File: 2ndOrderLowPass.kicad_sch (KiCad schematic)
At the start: 14 parts, among them U2 LM2904DR, U3 LM2904DR

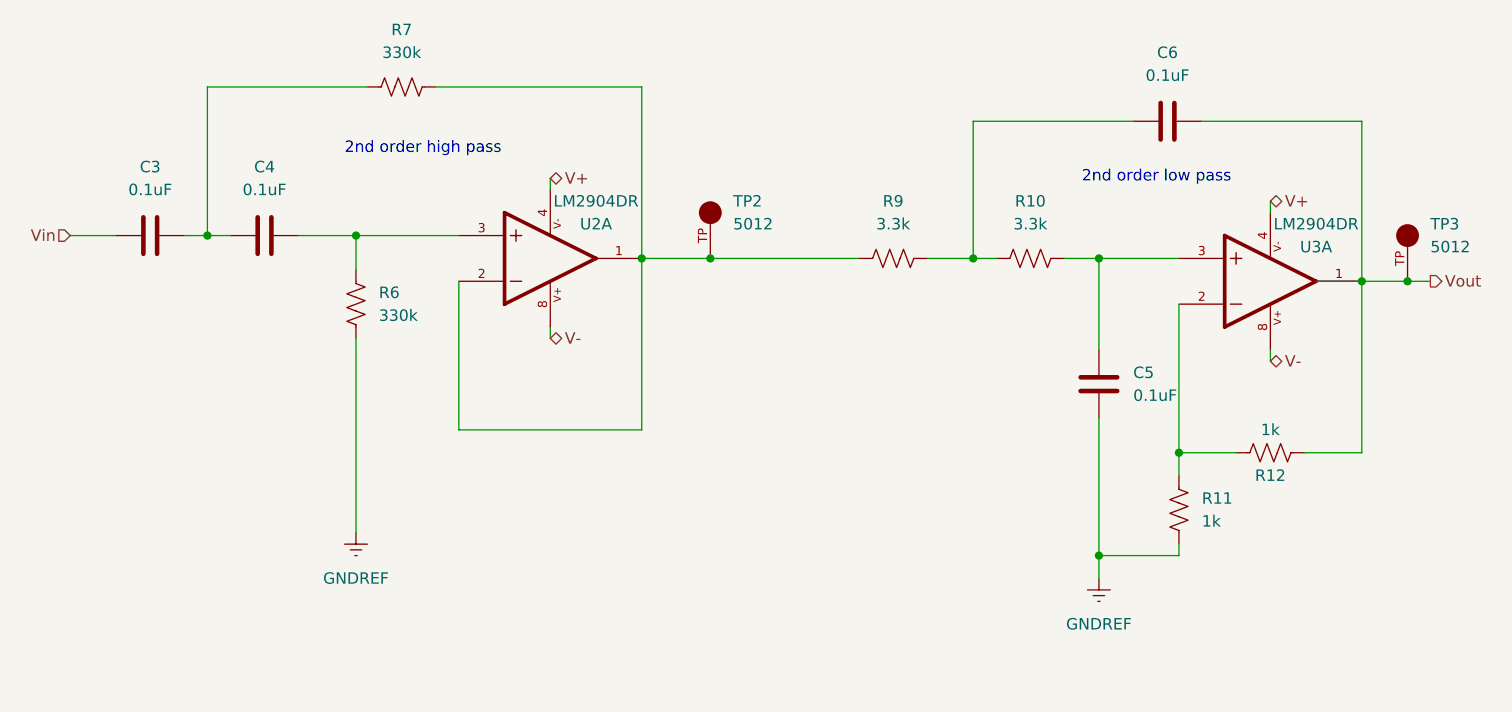
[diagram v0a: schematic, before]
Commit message: merge fix 2
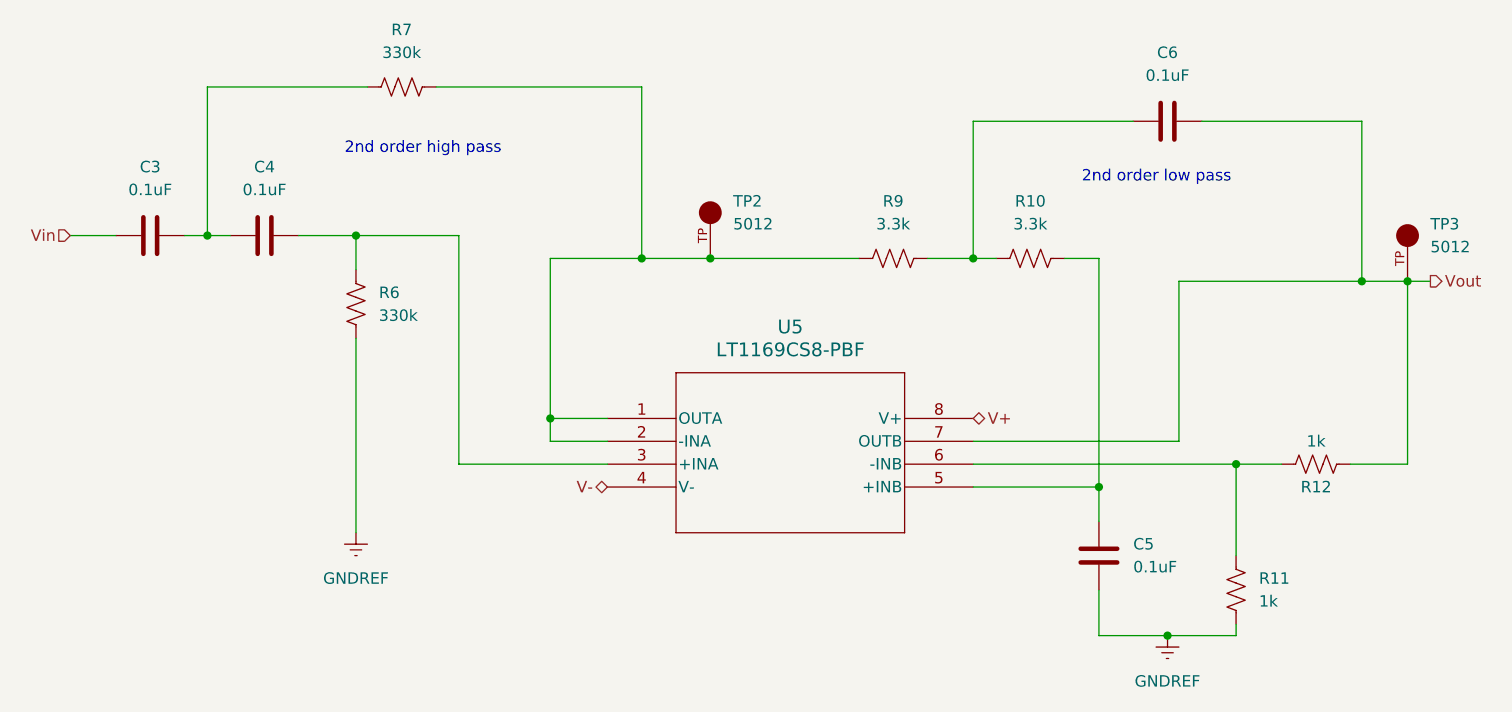
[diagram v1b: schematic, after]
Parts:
- removed U2, U3: LM2904DR, LM2904DR:SOIC127P599X175-8N, symbol Digikey2:LM2904DR
- added U5: LT1169CS8-PBF, SO-8_S_LIT, symbol symbols:LT1169CS8-PBF
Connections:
- net V+: now also U5.8 (V+)
- net V-: now also U5.4 (V-)
- net Vout: now also U5.7 (OUTB)
- net at R7.2, R9.2, TP2.TP: now also U5.1 (OUTA), U5.2 (-INA)
- net at R11.1, R12.1: now also U5.6 (-INB)
- net at C4.2, R6.1: now also U5.3 (+INA)
- net at C5.1, R10.2: now also U5.5 (+INB)
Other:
- moved on the sheet: C5, R11, R12
